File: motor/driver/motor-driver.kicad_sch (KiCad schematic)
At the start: 61 parts, among them J1 DEBUG, J2 sensors, J3 controller, J4 motor, J5 thermal, J6 external, U2 LM66100DCK, U4 TJA1051TK-3, U5 RP114x, U6 MCT8316Z-Q1, U7 CH32L103F8U6

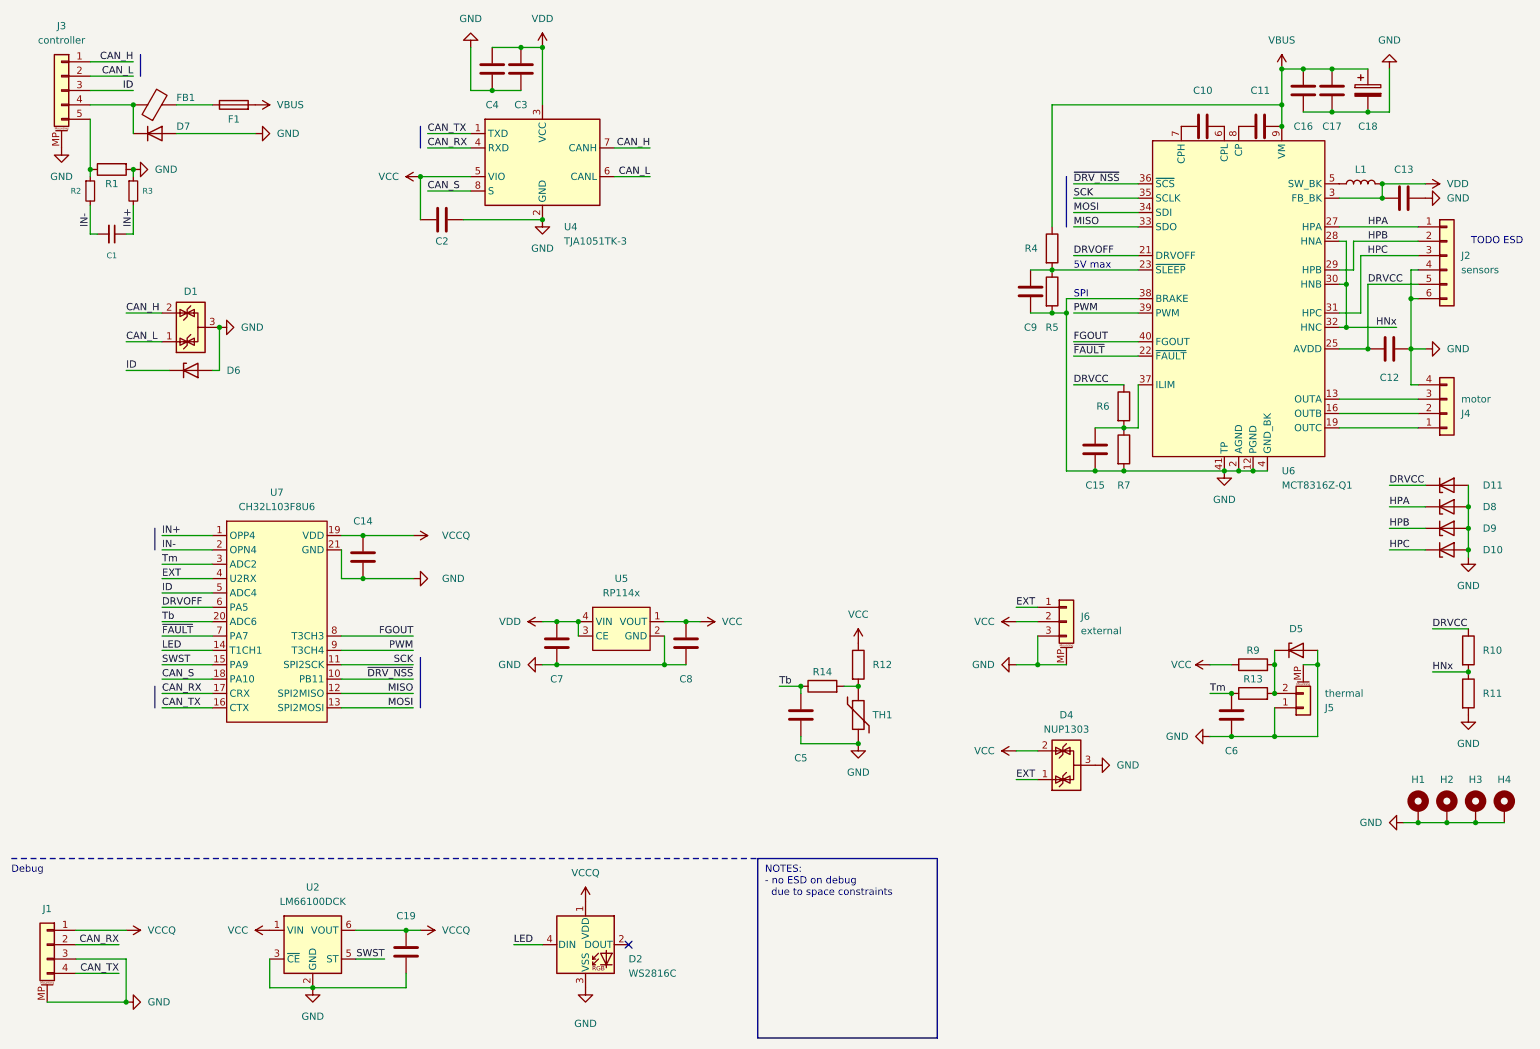
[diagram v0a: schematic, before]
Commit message: implement driver
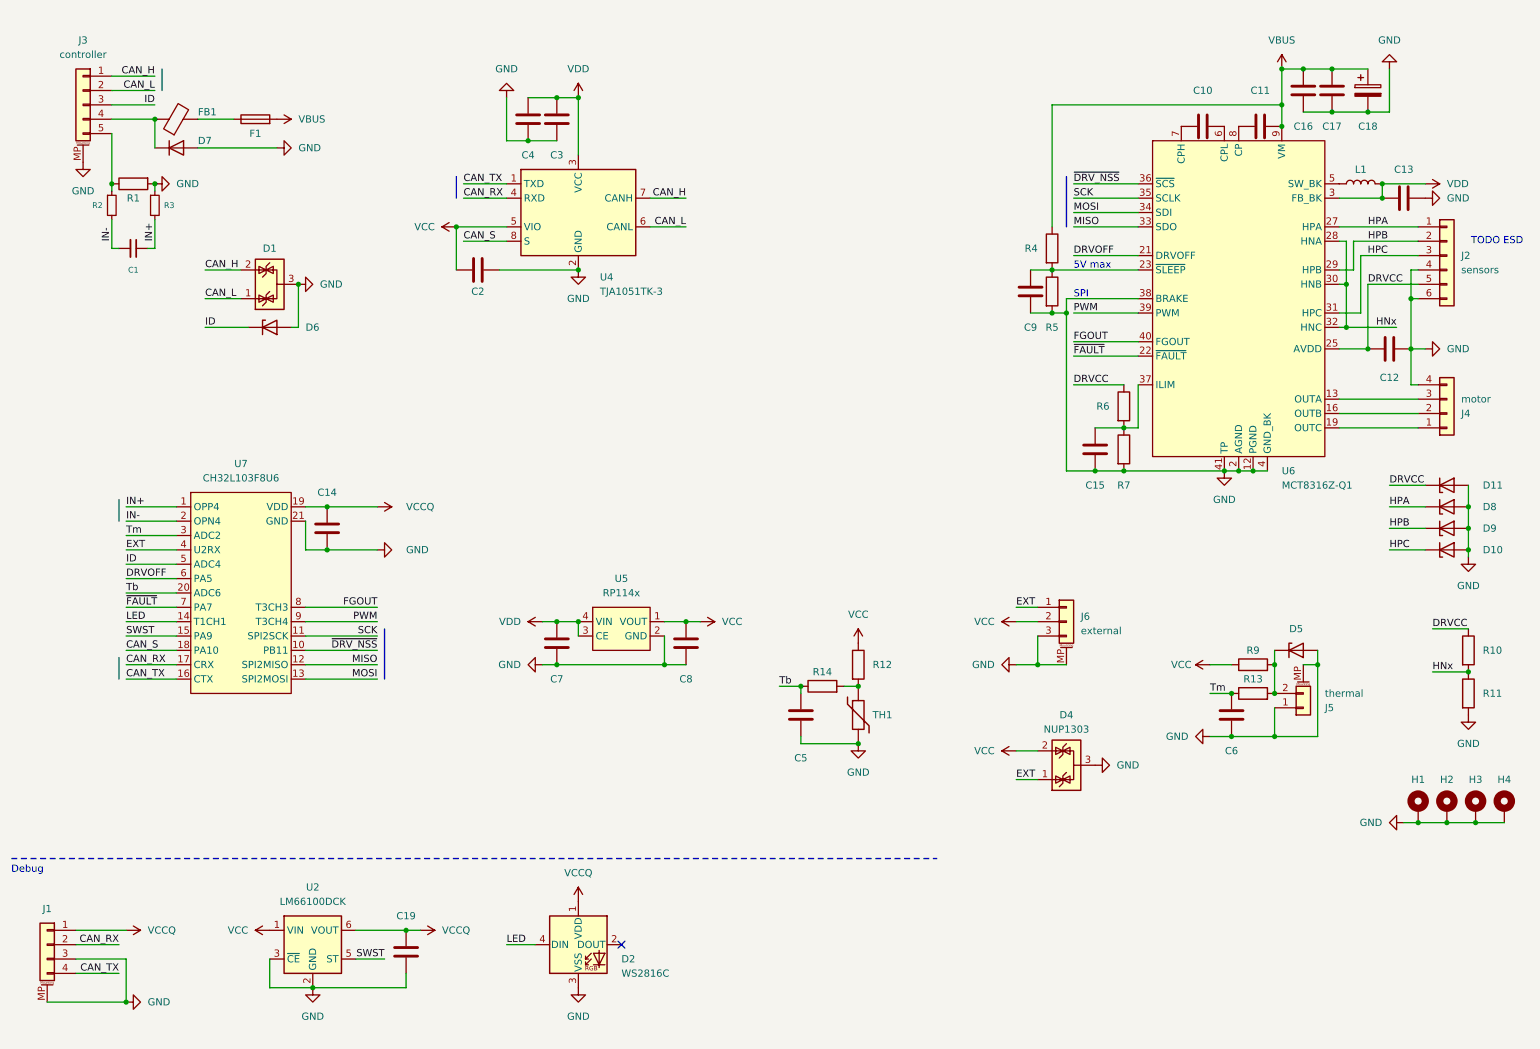
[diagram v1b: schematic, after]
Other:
- note removed: "NOTES: - no ESD on debug due to space constraints"
- moved on the sheet: C1, C14, C2, C3, C4, D1, D2, D6, D7, F1, FB1, J3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
